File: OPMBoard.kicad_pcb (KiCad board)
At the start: 2 copper layers, 80 x 60 mm, 35 parts, among them J1 USB_C_Receptacle_USB2.0, J2 Conn_01x03, J3 Conn_02x10_Counter_Clockwise, J4 AudioJack3, SW1 SW_SPDT, U1 NJM4580, U2 NJM4580, U4 YM2151, U5 YM3012, X1 CXO_DIP14, X2 CXO_DIP8

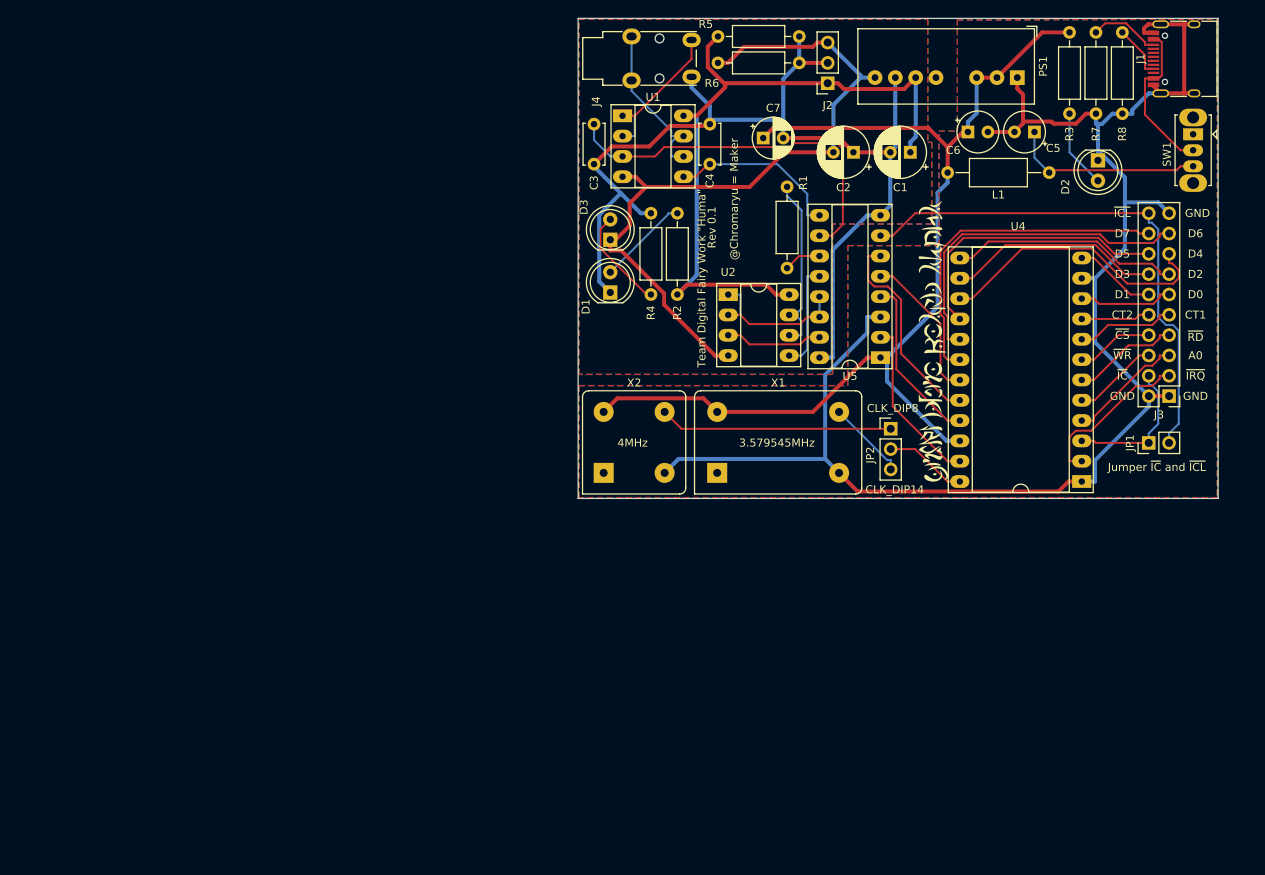
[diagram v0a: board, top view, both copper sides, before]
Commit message: Update schematic
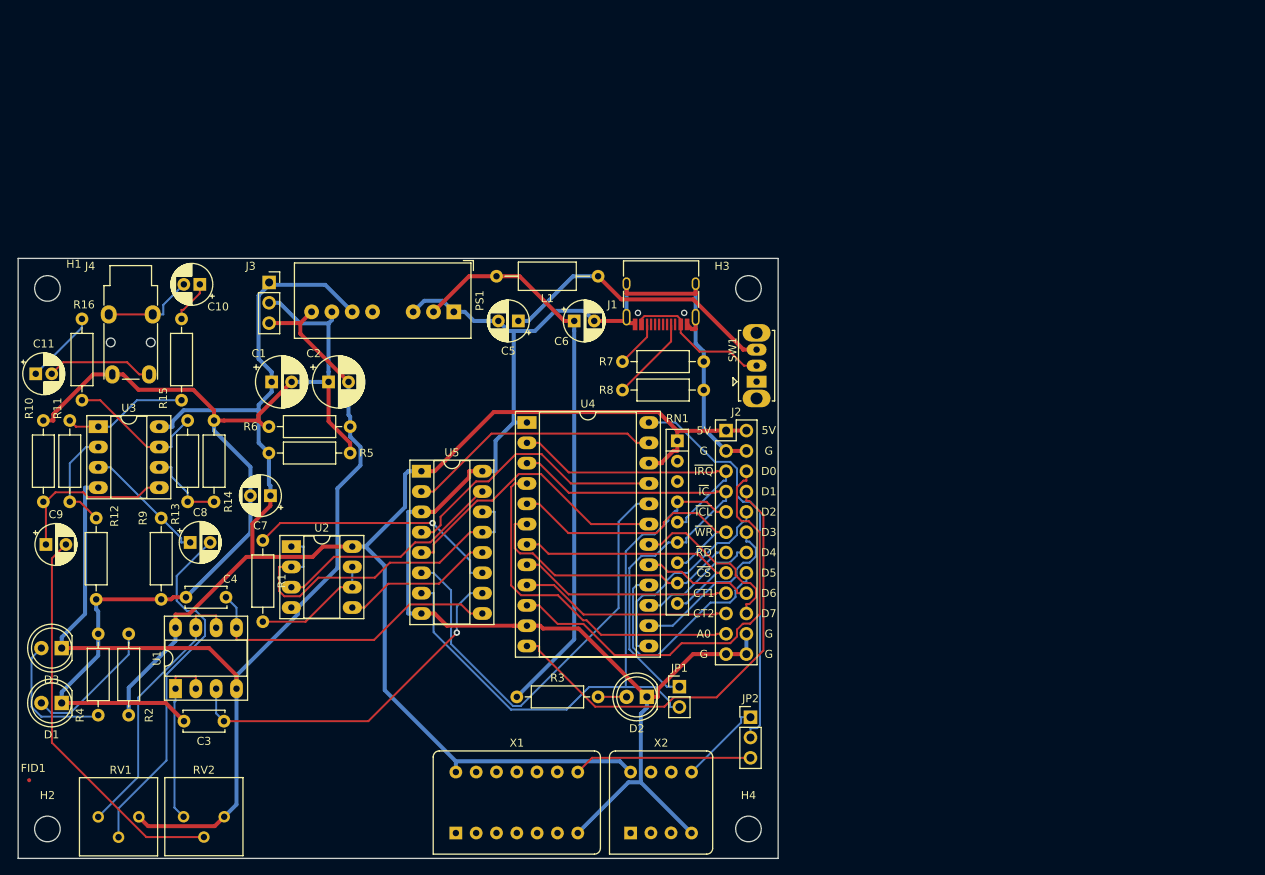
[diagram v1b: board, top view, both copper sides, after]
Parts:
- removed G*** (x2): LOGO, LOGO
- added C10: 470u, Capacitor_THT:CP_Radial_D5.0mm_P2.00mm, F.Cu at (92.7, 63.2)
- added C11: 470u, Capacitor_THT:CP_Radial_D5.0mm_P2.00mm, F.Cu at (72.2, 74.4)
- added C8: 10u, Capacitor_THT:CP_Radial_D5.0mm_P2.50mm, F.Cu at (91.5, 95.5)
- added C9: 10u, Capacitor_THT:CP_Radial_D5.0mm_P2.50mm, F.Cu at (73.5, 95.8)
- added FID1: Fiducial, Fiducial:Fiducial_0.5mm_Mask1mm, F.Cu at (71.4, 125.2)
- added H1: MountingHole, MountingHole:MountingHole_3.2mm_M3, F.Cu at (73.7, 63.8)
- added H2: MountingHole, MountingHole:MountingHole_3.2mm_M3, F.Cu at (73.7, 131.3)
- added H3: MountingHole, MountingHole:MountingHole_3.2mm_M3, F.Cu at (161.3, 63.8)
- added H4: MountingHole, MountingHole:MountingHole_3.2mm_M3, F.Cu at (161.3, 131.3)
- added R10: 10k, Resistor_THT:R_Axial_DIN0207_L6.3mm_D2.5mm_P10.16mm_Horizontal, F.Cu at (73.2, 90.4)
- added R11: 47k, Resistor_THT:R_Axial_DIN0207_L6.3mm_D2.5mm_P10.16mm_Horizontal, F.Cu at (76.5, 80.3)
- added R12: 10k, Resistor_THT:R_Axial_DIN0207_L6.3mm_D2.5mm_P10.16mm_Horizontal, F.Cu at (79.8, 92.5)
- added R13: 47k, Resistor_THT:R_Axial_DIN0207_L6.3mm_D2.5mm_P10.16mm_Horizontal, F.Cu at (91.2, 80.3)
- added R14: 10k, Resistor_THT:R_Axial_DIN0207_L6.3mm_D2.5mm_P10.16mm_Horizontal, F.Cu at (94.5, 90.4)
- added R15: 47, Resistor_THT:R_Axial_DIN0207_L6.3mm_D2.5mm_P10.16mm_Horizontal, F.Cu at (90.4, 77.7)
- added R16: 47, Resistor_THT:R_Axial_DIN0207_L6.3mm_D2.5mm_P10.16mm_Horizontal, F.Cu at (78.0, 77.7)
- added R9: 10k, Resistor_THT:R_Axial_DIN0207_L6.3mm_D2.5mm_P10.16mm_Horizontal, F.Cu at (87.9, 92.5)
- added RN1: 4.7k * 8, Resistor_THT:R_Array_SIP9, F.Cu at (152.4, 82.8)
- added RV1: 10kB, Potentiometer_THT:Potentiometer_Bourns_3386P_Vertical, F.Cu at (80.0, 129.8)
- added RV2: 10kB, Potentiometer_THT:Potentiometer_Bourns_3386P_Vertical, F.Cu at (90.7, 129.8)
- added U3: NJM4580, Package_DIP:DIP-8_W7.62mm_Socket_LongPads, F.Cu at (80.0, 81.0)
- C5, C6: footprint Capacitor_THT:CP_Radial_Tantal_D5.0mm_P2.50mm -> Capacitor_THT:CP_Radial_D5.0mm_P2.50mm
- D1: value 12V_GREEN -> 5V_GREEN
- D2: value 5V_GREEN -> VDD_GREEN
- D3: value -12V_GREEN -> -5V_GREEN
- J2: value Conn_01x03 -> Conn_02x12_Odd_Even; footprint Connector_PinSocket_2.54mm:PinSocket_1x03_P2.54mm_Vertical -> Connector_PinHeader_2.54mm:PinHeader_2x12_P2.54mm_Vertical
- J3: value Conn_02x10_Counter_Clockwise -> Conn_01x03; footprint Connector_PinHeader_2.54mm:PinHeader_2x10_P2.54mm_Vertical -> Connector_PinSocket_2.54mm:PinSocket_1x03_P2.54mm_Vertical
- PS1: value ITQ2415S -> ITX0505S-R
- R1: value 100 -> 270
- R2, R4: value 9.1k -> 2k
- X1: footprint Oscillator:Oscillator_DIP-14_LargePads -> MayLib:Oscillator_DIP-14_Full
- X2: footprint Oscillator:Oscillator_DIP-8_LargePads -> MayLib:Oscillator_DIP-8_Full
- moved J3 113.4 mm to (101.4, 63.0), turned to 0 degrees
- moved R3 108.0 mm to (132.3, 114.8), turned to 0 degrees
- moved U1 90.8 mm to (89.7, 113.8), turned to 90 degrees
- moved C3 87.8 mm to (95.7, 117.8), turned to 180 degrees
- moved D2 87.6 mm to (148.6, 114.8), turned to 180 degrees
- moved R4 86.8 mm to (80.0, 117.1)
- moved R2 86.4 mm to (83.8, 117.1)
- moved D1 85.6 mm to (75.4, 115.6), turned to 180 degrees
- moved D3 85.5 mm to (75.4, 108.7), turned to 180 degrees
- moved C1 84.8 mm to (101.7, 75.4), turned to 0 degrees
- moved C4 81.2 mm to (96.0, 102.4), turned to 180 degrees
- moved R6 80.4 mm to (101.3, 81.0), turned to 0 degrees
- moved R8 76.8 mm to (145.5, 76.5), turned to 0 degrees
- moved R5 76.6 mm to (101.3, 84.3)
- moved PS1 76.3 mm to (124.5, 66.7)
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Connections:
- C1 pad 1: +12V -> +5V
- C2 pad 2: -12V -> -5V
- C6 pad 1: +5V -> VDD
- D3 pad 1: -12V -> -5V
- J2 pad 1: +12V -> +5V
- J2 pad 2: GNDA -> +5V
- J2 pad 3: -12V -> GND
- J3 pad 1: GND -> +5V
- J3 pad 2: GND -> GNDA
- J3 pad 3: ~{IRQ} -> -5V
- L1 pad 2: +5V -> VDD
- PS1 pad 2: +5V -> VDD
- PS1 pad 3: +5V -> GND
- PS1 pad 6: +12V -> +5V
- PS1 pad 8: -12V -> -5V
- R2 pad 1: +12V -> +5V
- R3 pad 1: +5V -> VDD
- R5 pad 1: +12V -> +5V
- R6 pad 2: -12V -> -5V
- U1 pad 1: RCH_OUT -> RCH_FOLLOWER_OUT
- U1 pad 2: RCH_OUT -> RCH_FOLLOWER_OUT
- U1 pad 4: -12V -> -5V
- U1 pad 6: LCH_OUT -> LCH_FOLLOWER_OUT
- U1 pad 7: LCH_OUT -> LCH_FOLLOWER_OUT
- U1 pad 8: +12V -> +5V
- U2 pad 4: -12V -> -5V
- U2 pad 8: +12V -> +5V
- U5 pad 16: GNDA -> GND
- U5 pad 8: GNDA -> GND
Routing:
- net -5V: track 0.00 -> 138.1 mm
- net -12V: track 93.5 -> 0.00 mm
- net +5V: track 133.3 -> 225.4 mm
- net +12V: track 88.9 -> 0.00 mm
- net VDD: track 0.00 -> 71.7 mm
- net Net-(C9-Pad2): track 0.00 -> 49.4 mm
- net D1: track 10.3 -> 56.9 mm
- net Net-(C8-Pad2): track 0.00 -> 45.2 mm
- net ~{IC}: track 18.1 -> 61.9 mm
- net D0: track 11.9 -> 54.6 mm
- net CLK: track 10.3 -> 49.7 mm
- net LCH_FOLLOWER_OUT: track 0.00 -> 34.3 mm
- net SH1: track 26.2 -> 56.0 mm
- net A0: track 14.8 -> 43.9 mm
- net D6: track 42.8 -> 13.9 mm
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- removed copper zone on B.Cu, net GND
- removed copper zone on F.Cu, net GND
- removed copper zone on B.Cu, net GNDA
- removed copper zone on F.Cu, net GNDA
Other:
- board size 80 x 60 mm -> 95 x 75 mm
- board text added: "5V"
- board text added: "G"
- board text removed: "3.579545MHz"
- board text removed: "4MHz"
- board text removed: "@Chromaryu = Maker"
- board text removed: "CLK_DIP14"
- board text removed: "CLK_DIP8"
- board text removed: "GND"
- board text removed: "Jumper ~{IC} and ~{ICL}"
- board text removed: "Rev 0.1"
- board text removed: "Team Digital Fairy Work {dblquote}Huma{dblquote}"
